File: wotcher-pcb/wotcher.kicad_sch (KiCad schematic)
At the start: 105 parts, among them CN1 SM02B-SRSS-TB, SW1 SKTDLHE010, SW2 SKTDLHE010, SW3 SKTDLHE010, SW4 SKTDLHE010, U1 KCSA02-105, U2 KCSA02-105, U3 LIS2DW12TR-MS, U5 ATtiny1616-M, U6 KCSA02-105, U7 IS31FL3731-QF, U8 KCSA02-105, U9 DS3231MZ+

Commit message: added 3D model
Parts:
- U5: footprint Package_DFN_QFN:VQFN-20-1EP_3x3mm_P0.4mm_EP1.7x1.7mm -> easyeda2kicad:QFN-20_L3.0-W3.0-P0.40-BL-EP1.7
- U7: footprint Package_DFN_QFN:QFN-28-1EP_4x4mm_P0.4mm_EP2.3x2.3mm -> easyeda2kicad:QFN-28_L4.0-W4.0-P0.40-BL-EP
- W1, W10, W11, W12, W13, W14, W15, W16, W17, W18, W19, W2, W20, W21, W22, W23, W24, W25, W26, W27, W28, W29, W3, W30, W31, W32, W33, W34, W35, W36, W37, W38, W39, W4, W40, W41, W42, W43, W44, W45, W46, W47, W48, W49, W5, W50, W51, W52, W53, W54, W55, W56, W57, W58, W59, W6, W60, W61, W7, W8, W9: footprint ledproject:LED-SMD_L1.6-W0.8-R-RD -> easyeda2kicad:LED-SMD_L1.6-W0.8-R-RD

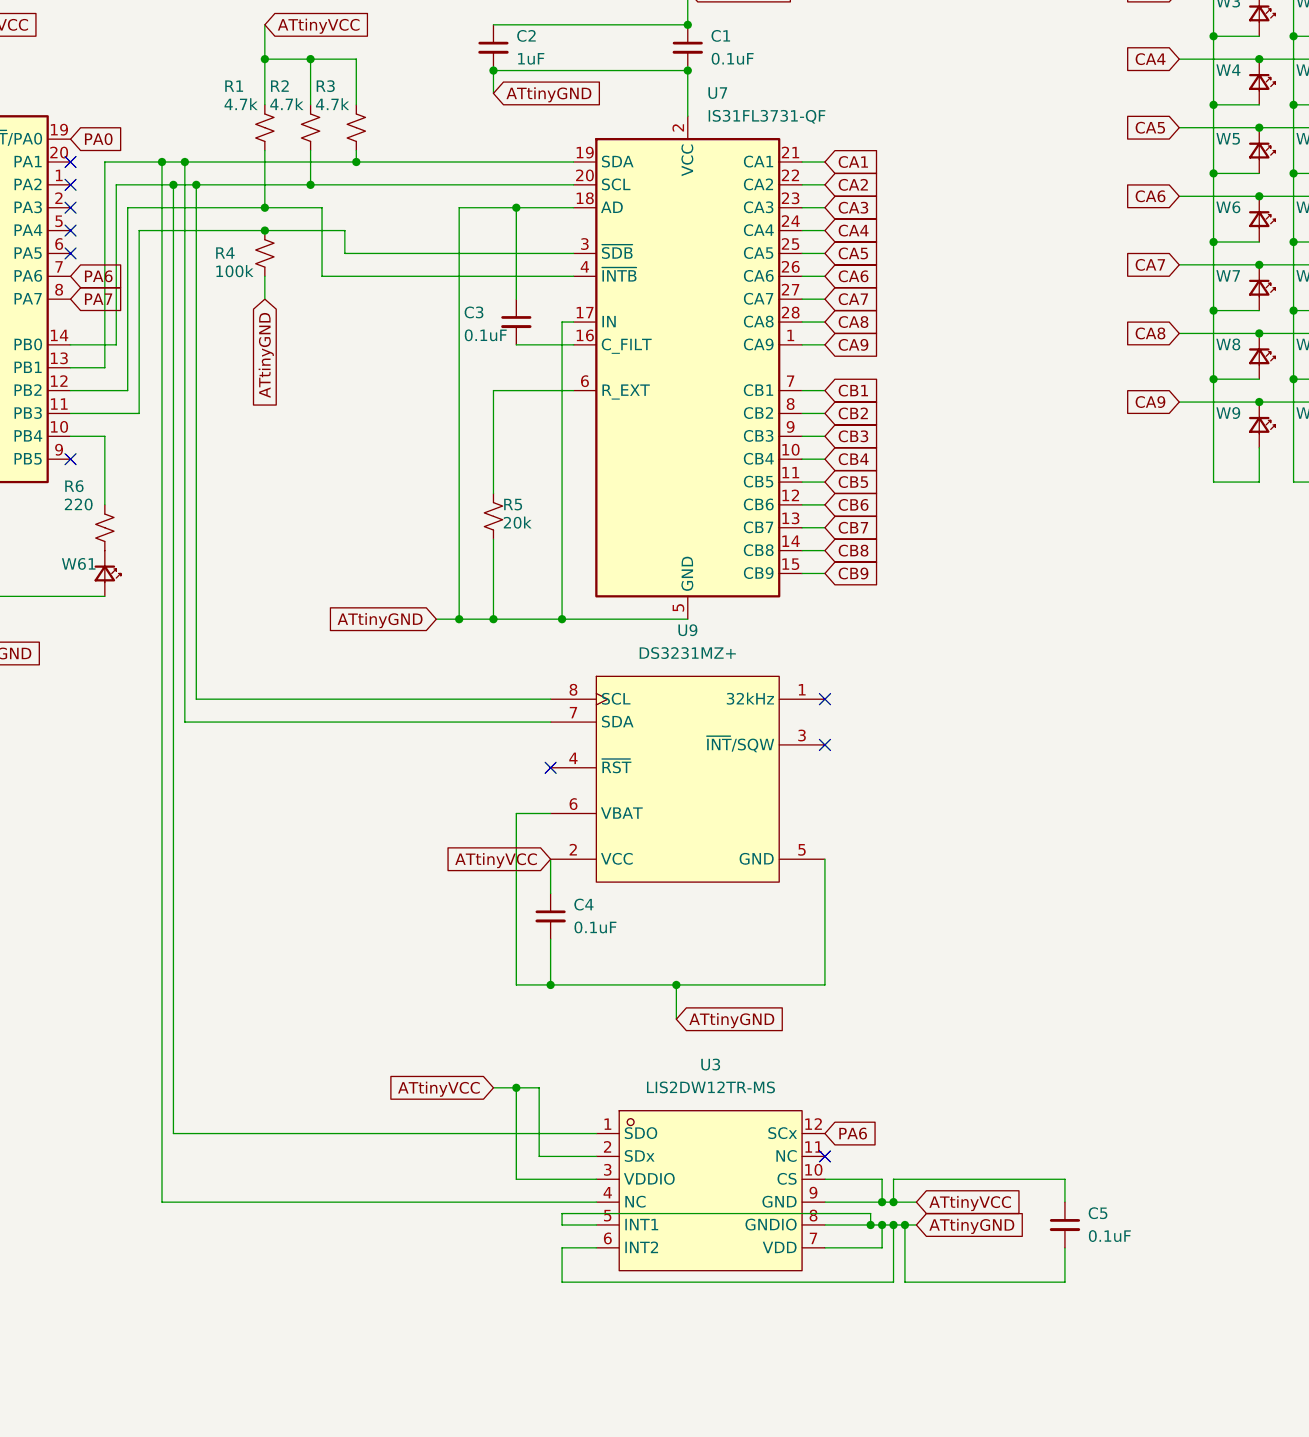
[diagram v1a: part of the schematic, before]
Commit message: re-wired something
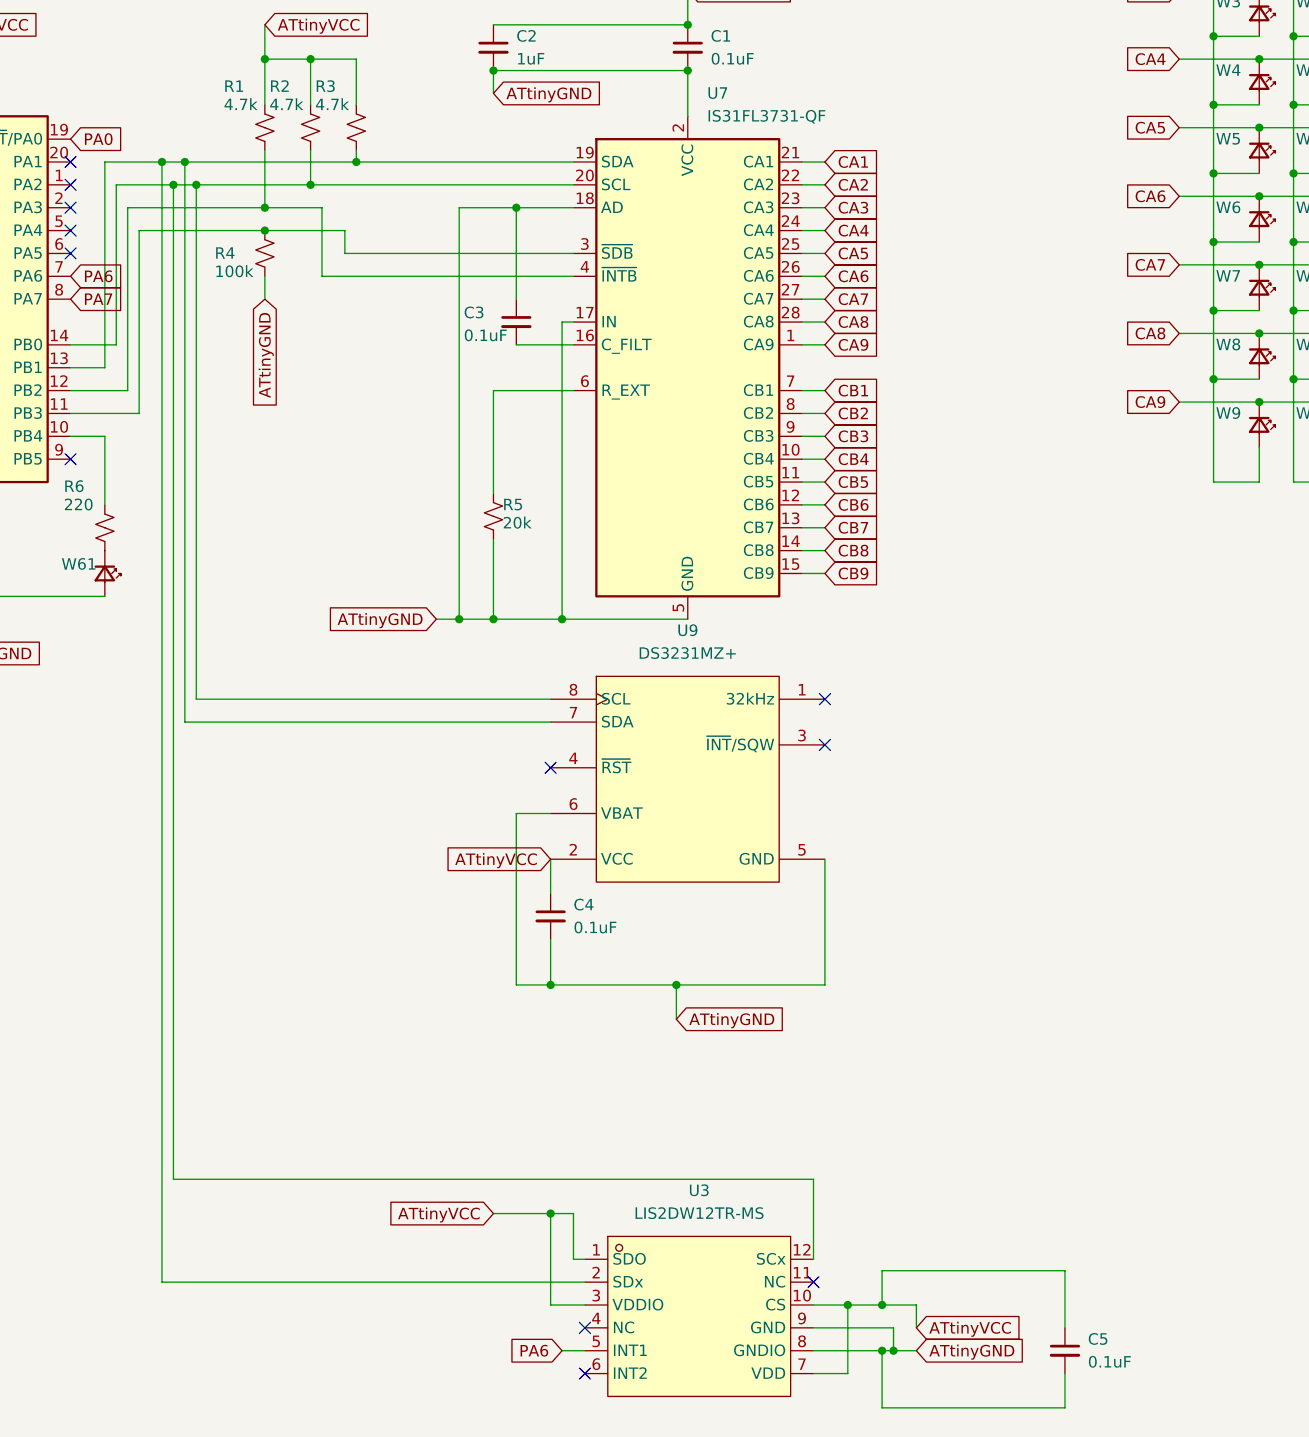
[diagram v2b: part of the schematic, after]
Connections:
- net +3: now also U3.1 (SDO), U3.7 (VDD); no longer U3.2 (SDx), U3.9 (GND)
- net GNDREF: now also U3.9 (GND); no longer U3.5 (INT1), U3.6 (INT2), U3.7 (VDD)
- net PA6: now also U3.5 (INT1); no longer U3.12 (SCx)
- net at R3.2, U5.13 (PB1), U7.19 (SDA)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: now also U3.2 (SDx); no longer U3.4 (NC)
- net at R2.2, U5.14 (PB0), U7.20 (SCL)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: now also U3.12 (SCx); no longer U3.1 (SDO)
- no-connect marks 10 -> 12
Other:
- moved on the sheet: C5, U3
